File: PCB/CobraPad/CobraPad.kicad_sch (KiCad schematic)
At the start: 35 parts, among them SW1 SW_Push, SW2 SW_Push, SW3 SW_Push, SW4 SW_Push, SW5 SW_Push, SW6 SW_Push, SW7 SW_Push, SW8 SW_Push, SW9 RotaryEncoder_Switch, U1 MOUDLE-SEEEDUINO-XIAO, U2 ER_OLEDM0.91_1x-I2C

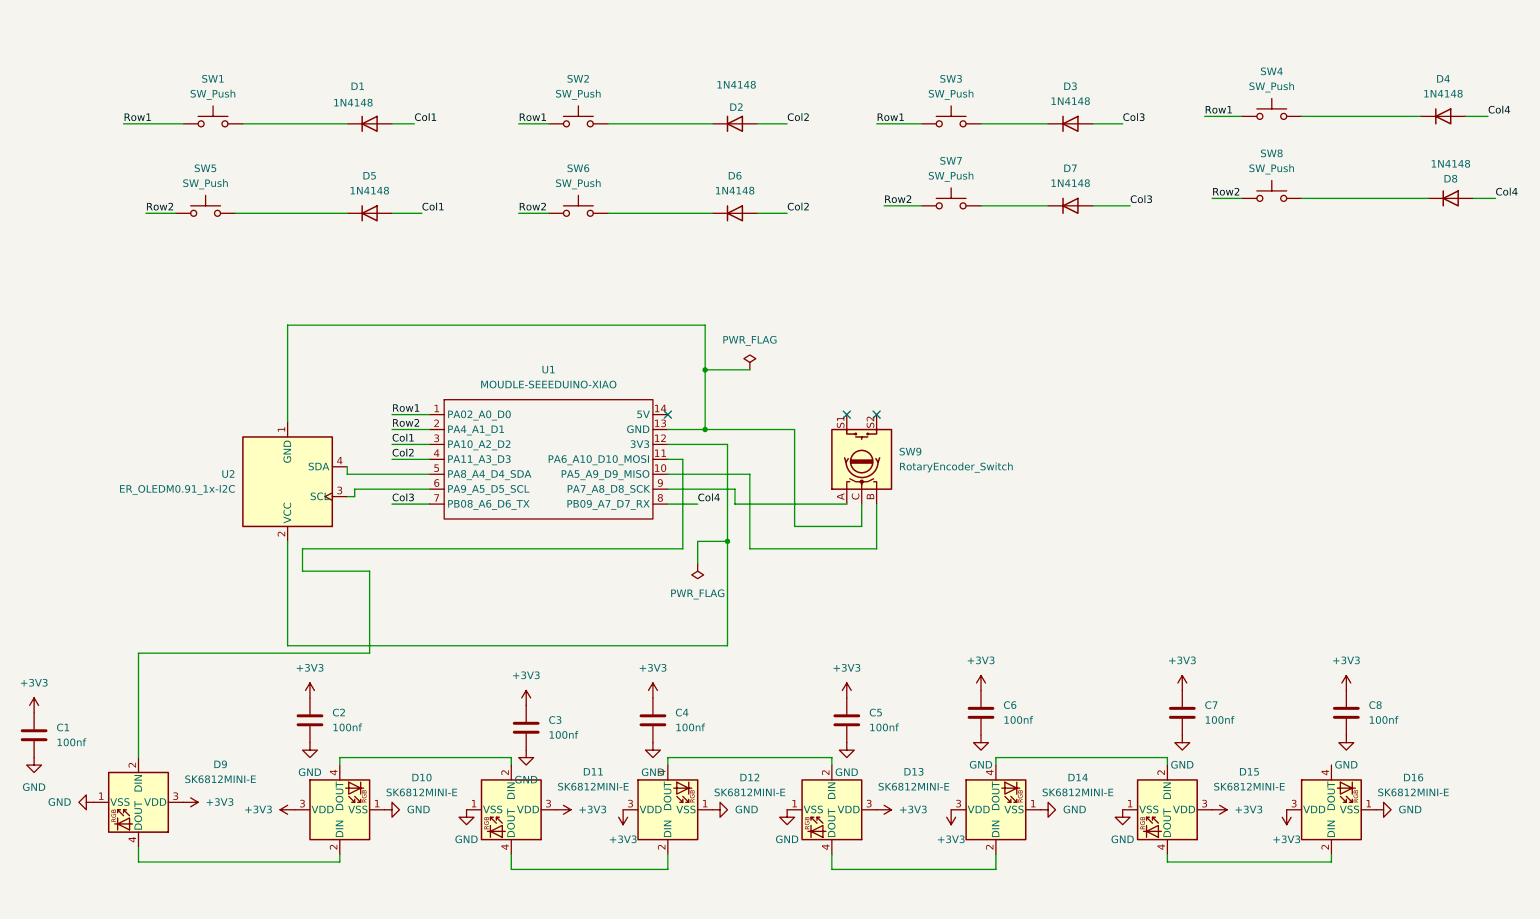
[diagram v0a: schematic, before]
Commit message: Fixed Keys
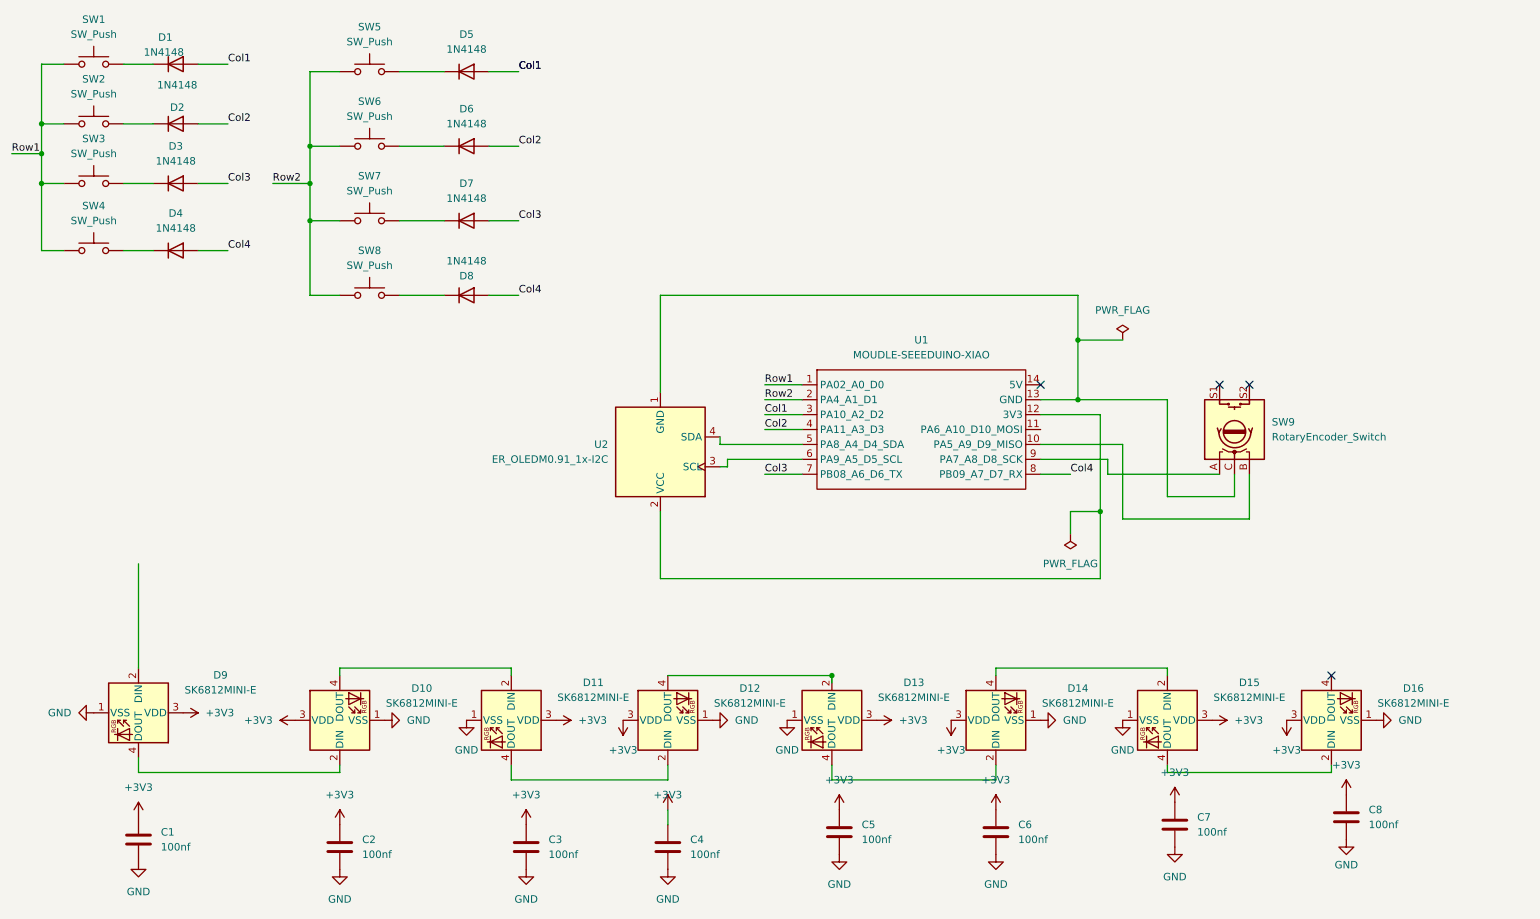
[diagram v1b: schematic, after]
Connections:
- net at D9.2 (DIN): no longer U1.11 (PA6_A10_D10_MOSI)
- no-connect marks 3 -> 4
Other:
- moved on the sheet: C1, C2, C3, C4, C5, C6, C7, C8, D1, D10, D11, D12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
